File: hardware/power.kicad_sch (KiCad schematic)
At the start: 35 parts, among them J14 Conn_01x02, Q11 AO3400A, Q12 DMP3013SFV, U5 TPS565208, U7 TPS82140SILR

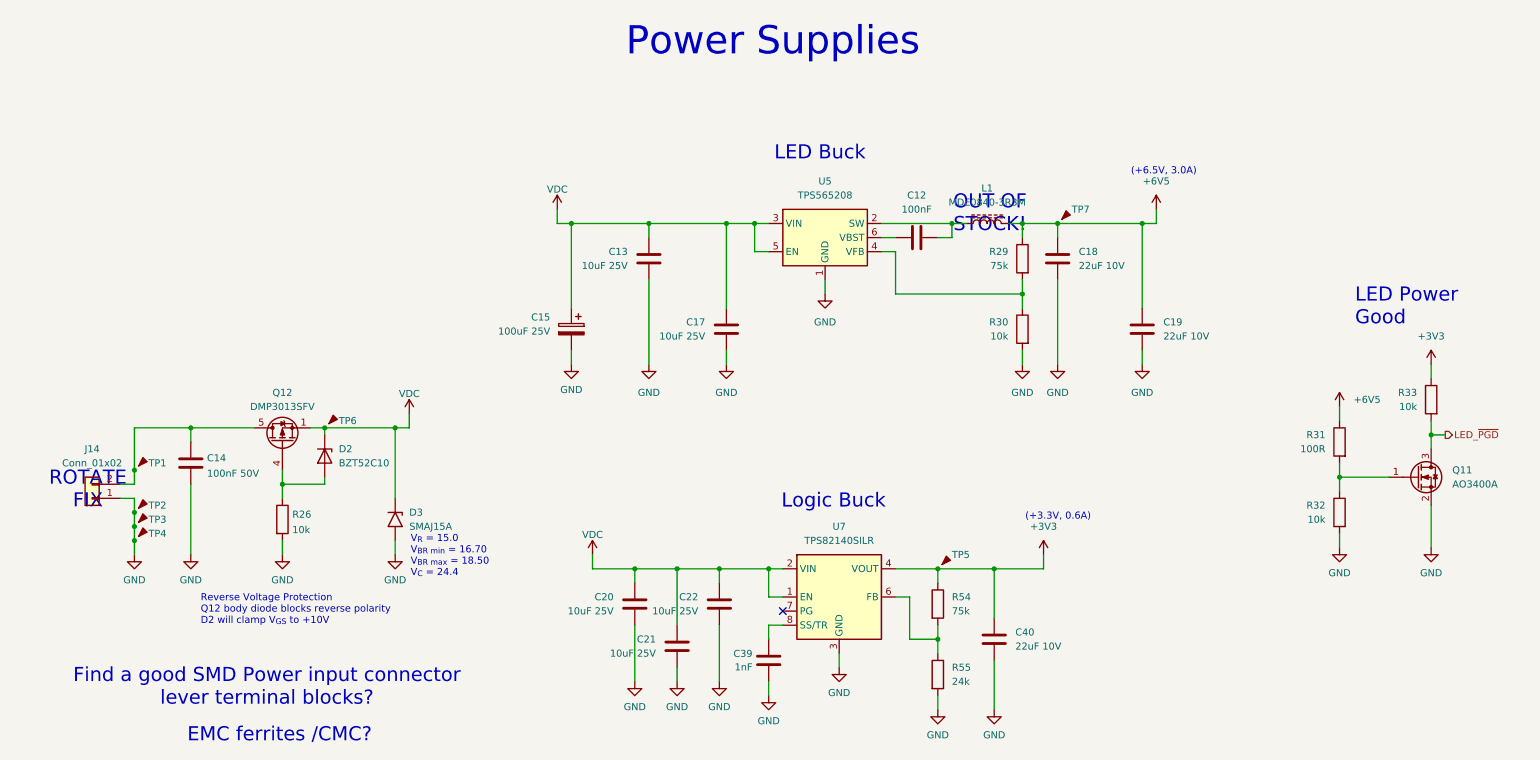
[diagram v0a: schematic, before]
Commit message: more layout and fixing OOS items
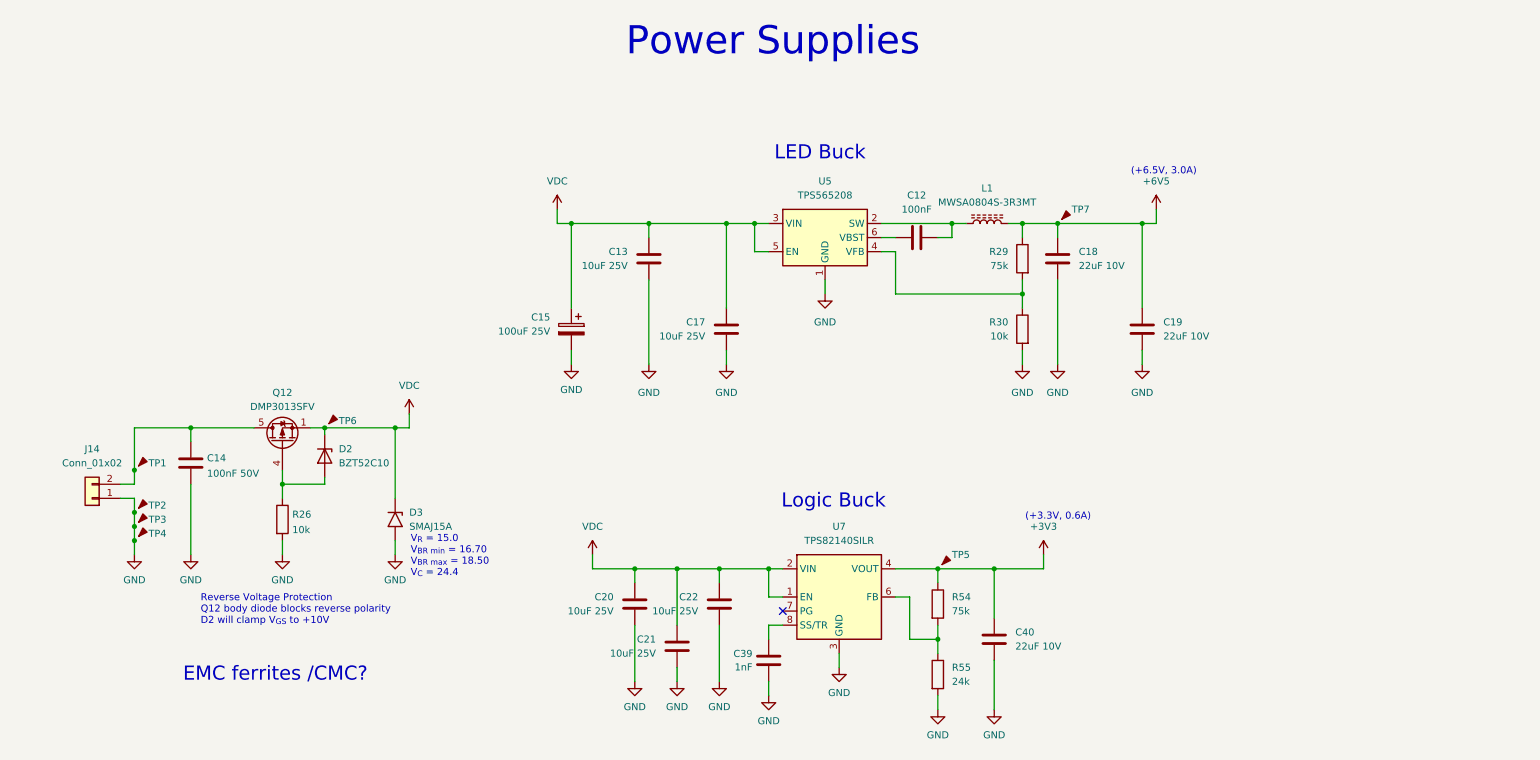
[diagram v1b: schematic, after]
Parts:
- removed Q11: AO3400A, Package_TO_SOT_SMD:SOT-23, symbol Transistor_FET:AO3400A
- removed R31: 100R, Resistor_SMD:R_0603_1608Metric, symbol Device:R
- removed R32, R33: 10k, Resistor_SMD:R_0603_1608Metric, symbol Device:R
- C12, C13, C14, C17, C18, C19, C20, C21, C22, C39, C40: symbol Device:C -> emf_beacon_ibrary:C
- C15: symbol Device:C_Polarized -> emf_beacon_ibrary:C_Polarized
- D2: symbol Device:D_Zener -> emf_beacon_ibrary:D_Zener
- D3: symbol Diode:SMAJ15A -> emf_beacon_ibrary:SMAJ15A
- J14: footprint TerminalBlock_WAGO:TerminalBlock_WAGO_2601-3102_1x02_P3.50mm_Vertical -> emf_beacon_library:MX250-3.5-02P-A-GY01-Cu-A; symbol Connector_Generic:Conn_01x02 -> emf_beacon_ibrary:Conn_01x02
- L1: value MDE0840-3R3M -> MWSA0804S-3R3MT; symbol Device:L_Ferrite -> emf_beacon_ibrary:L_Ferrite; LCSC C2875738 -> C17700166
- Q12: symbol Transistor_FET:DMP3013SFV -> emf_beacon_ibrary:DMP3013SFV
- R26, R29, R30, R54, R55: symbol Device:R -> emf_beacon_ibrary:R
- TP1, TP2, TP3, TP4, TP5, TP6, TP7: symbol Pinski1_Parts:TestPoint -> emf_beacon_ibrary:TestPoint
- U5: symbol Regulator_Switching:TPS565208 -> emf_beacon_ibrary:TPS565208
- U7: symbol Regulator_Switching:TPS82130 -> emf_beacon_ibrary:TPS82130
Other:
- note removed: "Find a good SMD Power input connector lever terminal blocks?"
- note removed: "LED Power Good"
- note removed: "OUT OF STOCK!"
- note removed: "ROTATE FIX"
